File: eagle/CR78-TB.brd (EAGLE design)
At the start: 100.8 x 80.8 mm, 39 parts, among them Q509 2N3904, Q522 2N3904, Q523 2N3904, Q524 2N3904, Q7 2N3904

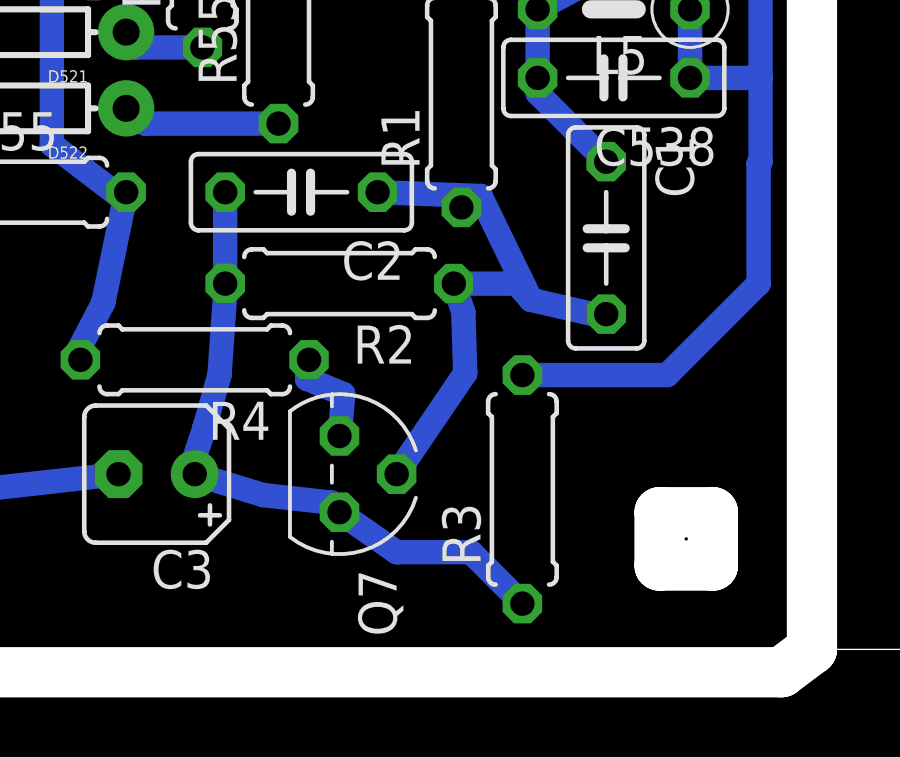
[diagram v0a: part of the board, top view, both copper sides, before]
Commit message: killed loose ends
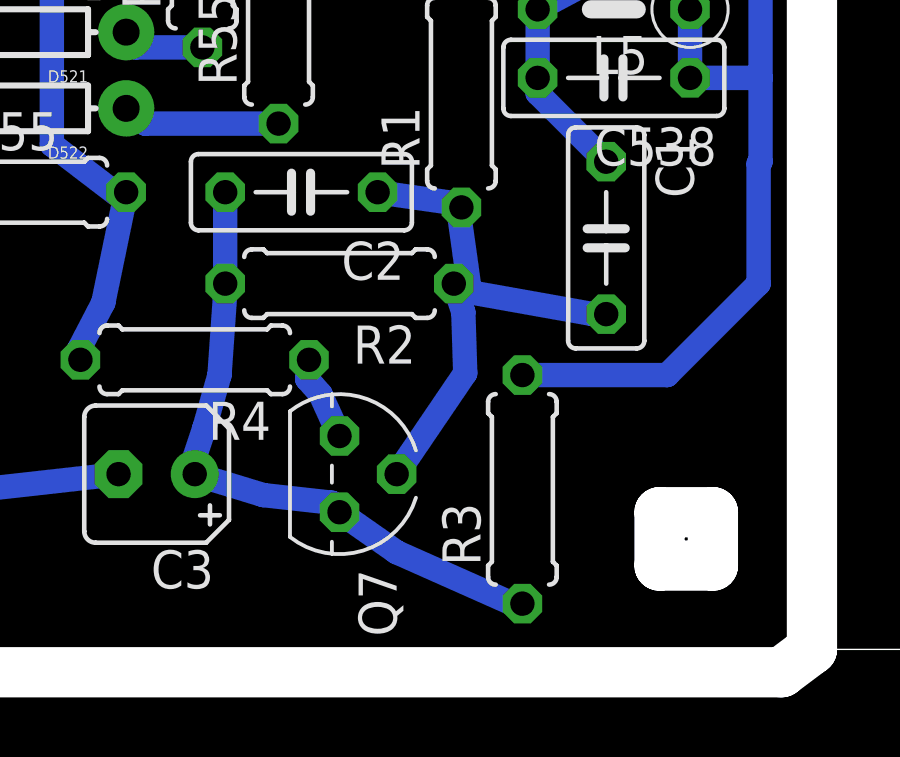
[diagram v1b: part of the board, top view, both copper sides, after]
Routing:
- net N$18: track 20.5 -> 18.5 mm
- net N$15: track 3.35 -> 2.85 mm
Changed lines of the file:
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@@
 <contactref element="Q7" pad="3"/>
 <contactref element="R4" pad="1"/>
-<wire x1="29.083" y1="8.509" x2="27.8765" y2="9.017" width="0.8128" layer="16"/>
-<wire x1="28.956" y1="7.112" x2="29.083" y2="8.509" width="0.8128" layer="16"/>
+<wire x1="28.321" y1="8.509" x2="27.8765" y2="9.017" width="0.8128" layer="16"/>
+<wire x1="28.956" y1="7.112" x2="28.321" y2="8.509" width="0.8128" layer="16"/>
 <wire x1="27.8765" y1="9.017" x2="27.94" y2="9.652" width="0.8128" layer="16"/>
 </signal>
@@
 <wire x1="24.0665" y1="6.223" x2="24.4475" y2="7.366" width="0.8128" layer="16"/>
 <wire x1="24.0665" y1="6.223" x2="24.13" y2="5.842" width="0.8128" layer="16"/>
-<wire x1="30.861" y1="3.2385" x2="33.3375" y2="3.2385" width="0.8128" layer="16"/>
-<wire x1="33.3375" y1="3.2385" x2="35.052" y2="1.524" width="0.8128" layer="16"/>
+<wire x1="30.861" y1="3.2385" x2="34.8615" y2="1.4605" width="0.8128" layer="16"/>
+<wire x1="34.8615" y1="1.4605" x2="35.052" y2="1.524" width="0.8128" layer="16"/>
 </signal>
 <signal name="N$18">
@@
 <wire x1="33.147" y1="9.2075" x2="30.861" y2="5.842" width="0.8128" layer="16"/>
 <wire x1="37.4015" y1="11.176" x2="37.846" y2="11.176" width="0.8128" layer="16"/>
-<wire x1="34.8615" y1="12.192" x2="35.33775" y2="11.65225" width="0.8128" layer="16"/>
-<wire x1="35.33775" y1="11.65225" x2="37.4015" y2="11.176" width="0.8128" layer="16"/>
-<wire x1="34.8615" y1="12.192" x2="32.766" y2="12.192" width="0.8128" layer="16"/>
-<wire x1="35.33775" y1="11.65225" x2="33.655" y2="15.113" width="0.8128" layer="16"/>
-<wire x1="33.655" y1="15.113" x2="30.226" y2="15.24" width="0.8128" layer="16"/>
-<wire x1="33.655" y1="15.113" x2="33.02" y2="14.732" width="0.8128" layer="16"/>
+<wire x1="32.8295" y1="12.446" x2="33.30575" y2="11.90625" width="0.8128" layer="16"/>
+<wire x1="33.30575" y1="11.90625" x2="37.4015" y2="11.176" width="0.8128" layer="16"/>
+<wire x1="32.8295" y1="12.446" x2="32.766" y2="12.192" width="0.8128" layer="16"/>
+<wire x1="33.30575" y1="11.90625" x2="32.893" y2="14.859" width="0.8128" layer="16"/>
+<wire x1="32.893" y1="14.859" x2="30.226" y2="15.24" width="0.8128" layer="16"/>
+<wire x1="32.893" y1="14.859" x2="33.02" y2="14.732" width="0.8128" layer="16"/>
 </signal>
 <signal name="N$19">
